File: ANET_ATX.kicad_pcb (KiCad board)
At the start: 2 copper layers, 65 x 56 mm, 16 parts, among them J1 External connect, J4 39357-0002, J5 39357-0002, Q1 2N3904

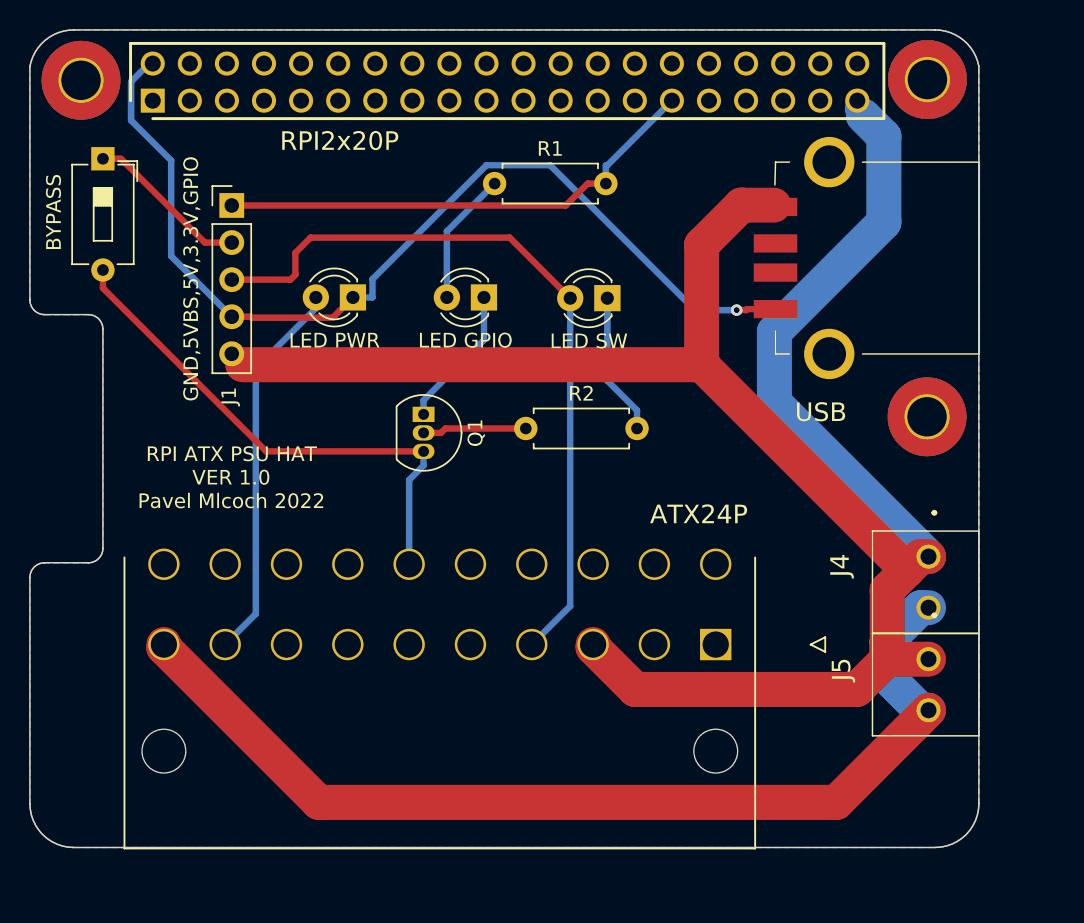
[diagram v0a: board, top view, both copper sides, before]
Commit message: replaced best parts
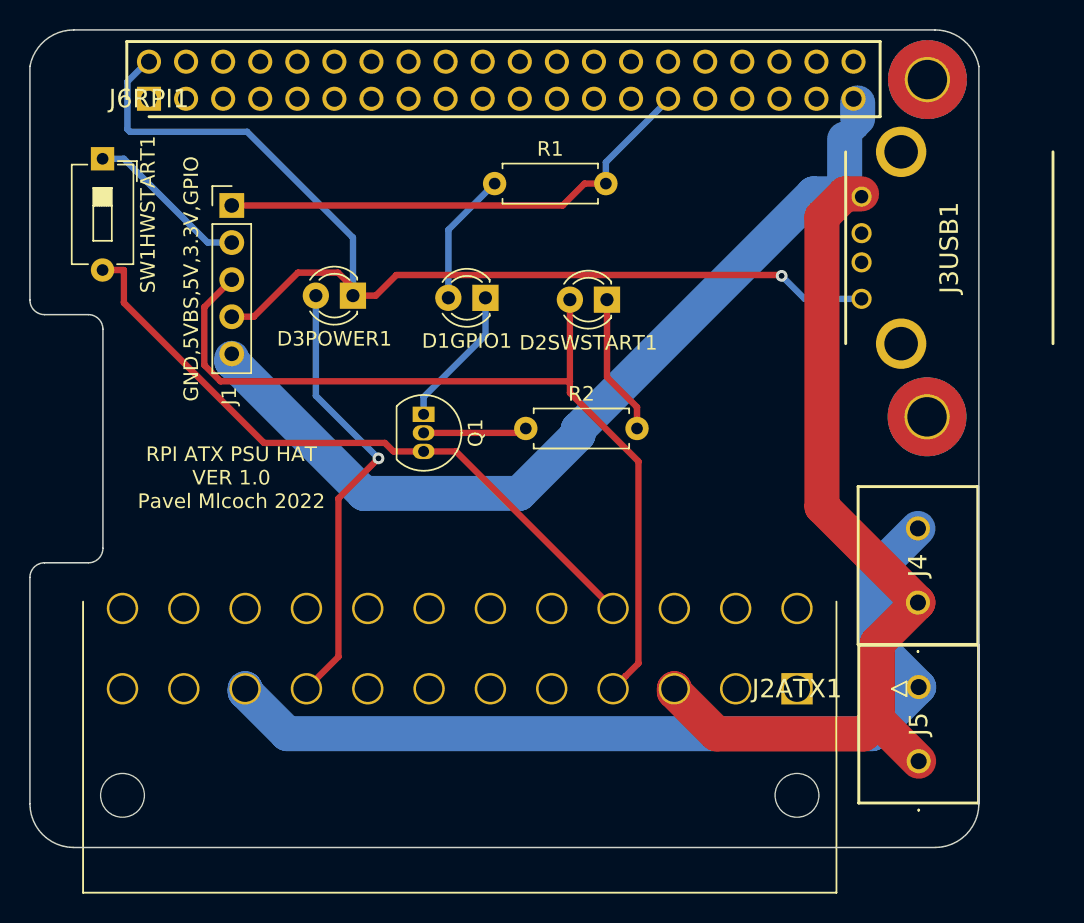
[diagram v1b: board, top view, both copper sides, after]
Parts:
- removed ATX24P: 39-30-1200, SamacSys_Parts:39-30-120Y_012
- removed BYPASS: SW_DIP_x01, Button_Switch_THT:SW_DIP_SPSTx01_Slide_6.7x4.1mm_W7.62mm_P2.54mm_LowProfile
- removed H2: H2, MountingHole:MountingHole_2.7mm_M2.5_Pad_TopBottom
- removed LED GPIO: 1N4003, LED_THT:LED_D3.0mm
- removed LED PWR: 1N4003, LED_THT:LED_D3.0mm
- removed LED SW: 1N4003, LED_THT:LED_D3.0mm
- removed RPI2x20P: BLG2X20, SamacSys_Parts:RHDR40W64P254X254_2X20_5130X500X865P
- removed USB: 292303-7, SamacSys_Parts:2923037
- added D1GPIO1: 1N4003, LED_THT:LED_D3.0mm, F.Cu at (79.2, 78.3)
- added D2SWSTART1: 1N4003, LED_THT:LED_D3.0mm, F.Cu at (87.5, 78.4)
- added D3POWER1: 1N4003, LED_THT:LED_D3.0mm, F.Cu at (70.1, 78.1)
- added J2ATX1: 39-30-1240, SamacSys_Parts:39-30-124Y_012, F.Cu at (100.5, 105.1)
- added J3USB1: 292303-7, SamacSys_Parts:A-USBSA, F.Cu at (111.0, 74.8)
- added J6RPI1: BLG2X20, SamacSys_Parts:RHDR40W64P254_2X20_5130X500X1375P, F.Cu at (56.1, 64.6)
- added SW1HWSTART1: SW_DIP_x01, Button_Switch_THT:SW_DIP_SPSTx01_Slide_6.7x4.1mm_W7.62mm_P2.54mm_LowProfile, F.Cu at (53.0, 68.8)
- J4, J5: footprint SamacSys_Parts:393570002 -> SamacSys_Parts:0398800302
- moved J5 7.02 mm to (108.8, 110.0), turned to 90 degrees
- moved J4 3.23 mm to (108.8, 99.2), turned to 90 degrees
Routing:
- net GND: track 140.0 -> 124.8 mm
- net +5V: track 51.8 -> 62.7 mm
- net Net-(J2ATX1-Pad16): track 36.0 -> 45.9 mm
- net 12V: track 69.6 -> 62.1 mm
- net 5VSB: track 67.4 -> 74.4 mm
- net Net-(D3POWER1-Pad2): track 26.3 -> 30.7 mm, vias 0 -> 1
- removed copper zone on B.Cu, net GND
- removed copper zone on F.Cu, net GND
